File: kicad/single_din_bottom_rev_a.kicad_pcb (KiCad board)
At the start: 2 copper layers, 86 x 14 mm, 9 parts, among them J1 Conn_01x04, J2 Conn_01x04, J3 Conn_01x04, J4 Conn_01x04, U1 R-78B3.3-1.0 (Recom)

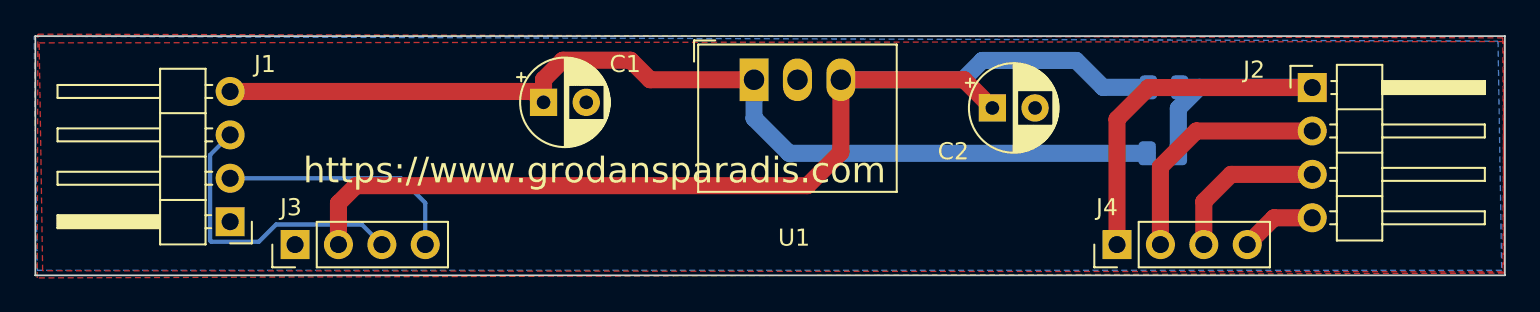
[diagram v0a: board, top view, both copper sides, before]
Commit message: Added cutots
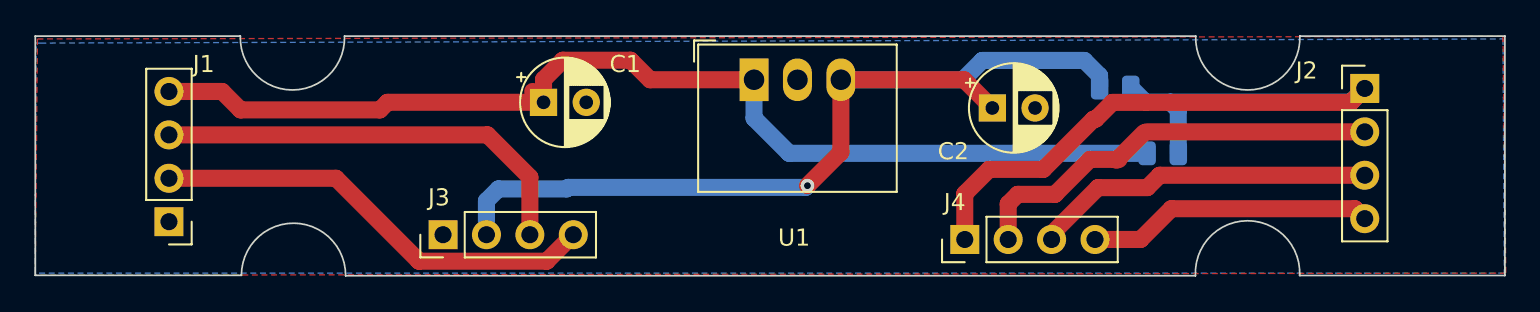
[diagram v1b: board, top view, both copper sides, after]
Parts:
- J1, J2: footprint Connector_PinHeader_2.54mm:PinHeader_1x04_P2.54mm_Horizontal -> Connector_PinHeader_2.54mm:PinHeader_1x04_P2.54mm_Vertical
- moved J4 8.91 mm to (84.4, 177.9)
- moved J3 8.68 mm to (53.9, 177.6)
- moved J1 3.58 mm to (37.8, 176.9)
- moved J2 3.07 mm to (107.8, 169.1)
- moved R1 2.86 mm to (93.2, 169.0)
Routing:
- net /IO1: track 31.7 -> 46.4 mm
- net /IO4: track 4.45 -> 16.8 mm
- net Net-(J1-Pad2): track 14.5 -> 26.3 mm
- net /Vout: track 66.0 -> 54.4 mm, vias 0 -> 1
- net /IO3: track 9.52 -> 20.1 mm
- net /IO2: track 14.3 -> 24.8 mm
- net Net-(J1-Pad3): track 17.7 -> 25.5 mm
- net /Vin: track 59.3 -> 64.1 mm
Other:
- outline, holes or cut-outs redrawn
- board text added: "DIN M1 Base board rev B"
- board text removed: "DIN M1 Base board rev A"
